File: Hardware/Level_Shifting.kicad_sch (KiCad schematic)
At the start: 45 parts, among them J12 SMA_Edge, J3 SMA_Edge, SW4 DPDT_Slide_SMD_7.2x3.5mm, U10 74LVC2T45DC, U12 74LVC2T45DC, U16 74LVC2T45DC, U18 PCA9306, U8 74LVC2T45DC, U9 74LVC2T45DC

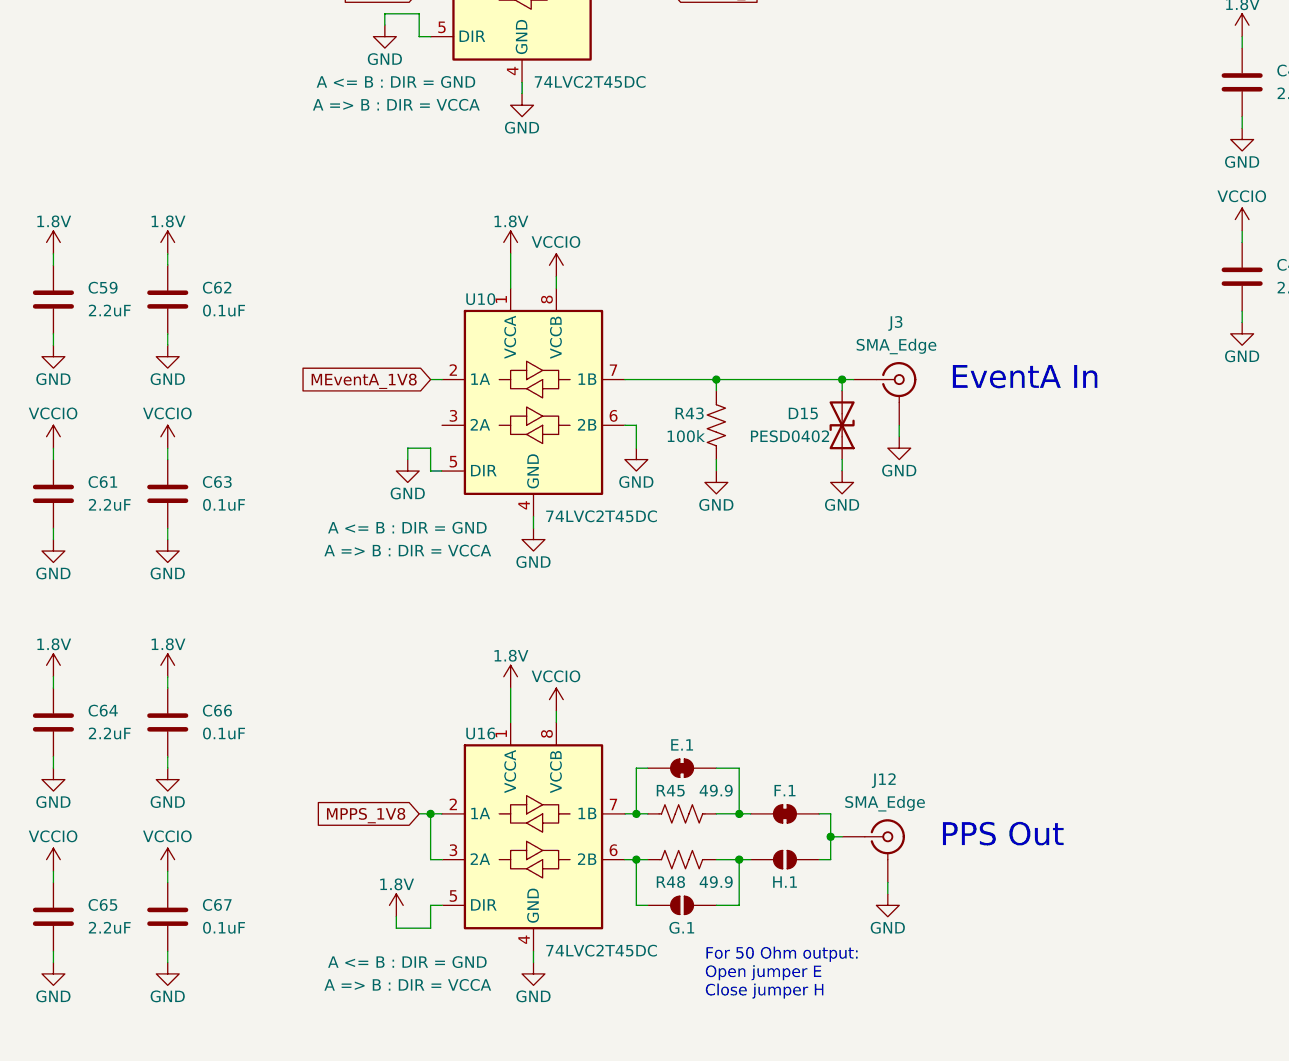
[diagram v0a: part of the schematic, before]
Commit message: Add jumpers for 2.8V and 1.8V In / Out
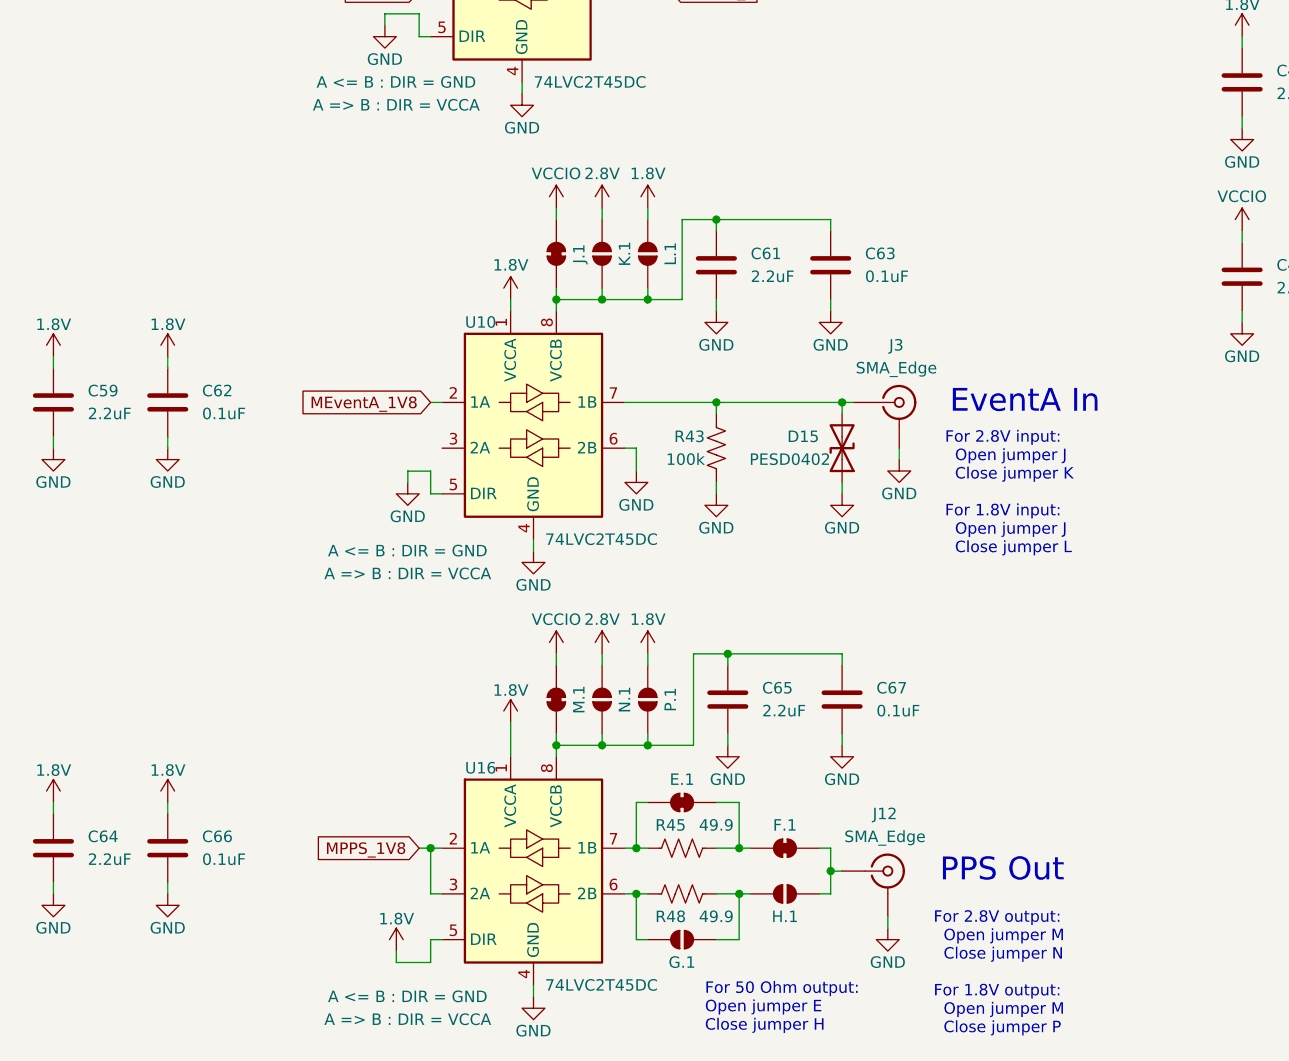
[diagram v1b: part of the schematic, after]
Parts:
- added J.1, M.1: ~, SparkFun-Jumper:Jumper_2_NC_Trace, symbol SparkFun-Jumper:SolderJumper_2_Bridged
- added K.1, L.1, N.1, P.1: ~, SparkFun-Jumper:Jumper_2_NO, symbol SparkFun-Jumper:SolderJumper_2_Open
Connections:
- net 1.8V: now also L.1.2 (B), P.1.2 (B)
- net VCCIO: now also J.1.2 (B), M.1.2 (B); no longer C61.1, C63.1, C65.1, C67.1, U10.8 (VCCB), U16.8 (VCCB)
- new net: C65.1, C67.1, M.1.1 (A), N.1.1 (A), P.1.1 (A), U16.8 (VCCB)
- new net: C61.1, C63.1, J.1.1 (A), K.1.1 (A), L.1.1 (A), U10.8 (VCCB)
- new net 2.8V: K.1.2 (B), N.1.2 (B)
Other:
- note added: "For 2.8V input: Open jumper J Close jumper K For 1.8V input: Open jumper J Close jumper L"
- note added: "For 2.8V output: Open jumper M Close jumper N For 1.8V output: Open jumper M Close jumper P"
- moved on the sheet: C59, C61, C62, C63, C64, C65, C66, C67, D15, E.1, F.1, G.1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
